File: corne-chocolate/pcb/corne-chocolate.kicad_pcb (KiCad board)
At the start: 2 copper layers, 133.8 x 91.4 mm, 98 parts, among them J3 LED, P1 i2c-pin, P2 i2c-pin, SW1 SW_PUSH, SW10 SW_PUSH, SW11 SW_PUSH, SW12 SW_PUSH, SW13 SW_PUSH, SW14 SW_PUSH, SW15 SW_PUSH, SW16 SW_PUSH, SW17 SW_PUSH, SW18 SW_PUSH, SW19 SW_PUSH, SW2 SW_PUSH, SW20 SW_PUSH, SW21 SW_PUSH, SW3 SW_PUSH, SW4 SW_PUSH, SW5 SW_PUSH, SW6 SW_PUSH, SW7 SW_PUSH, SW8 SW_PUSH, SW9 SW_PUSH, U1 ProMicro

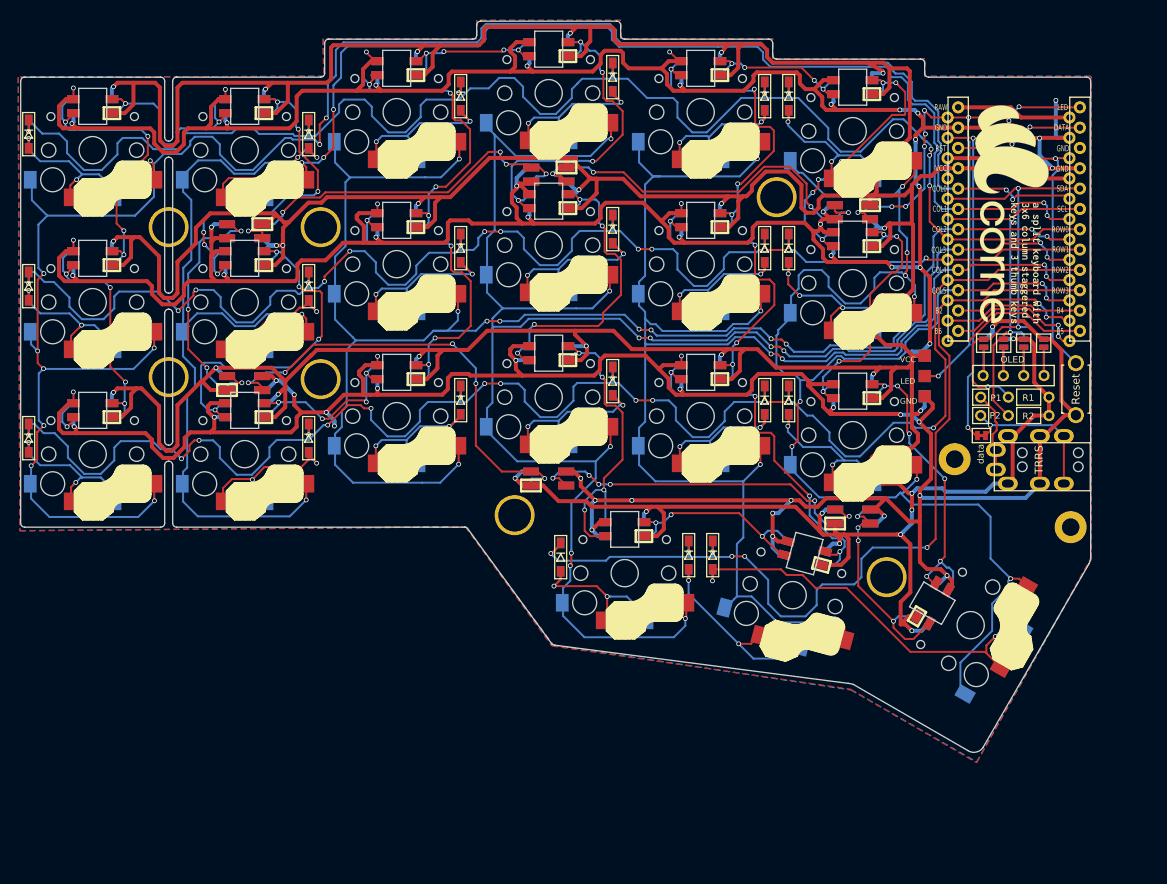
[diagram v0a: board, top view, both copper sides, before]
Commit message: rp2040 v0
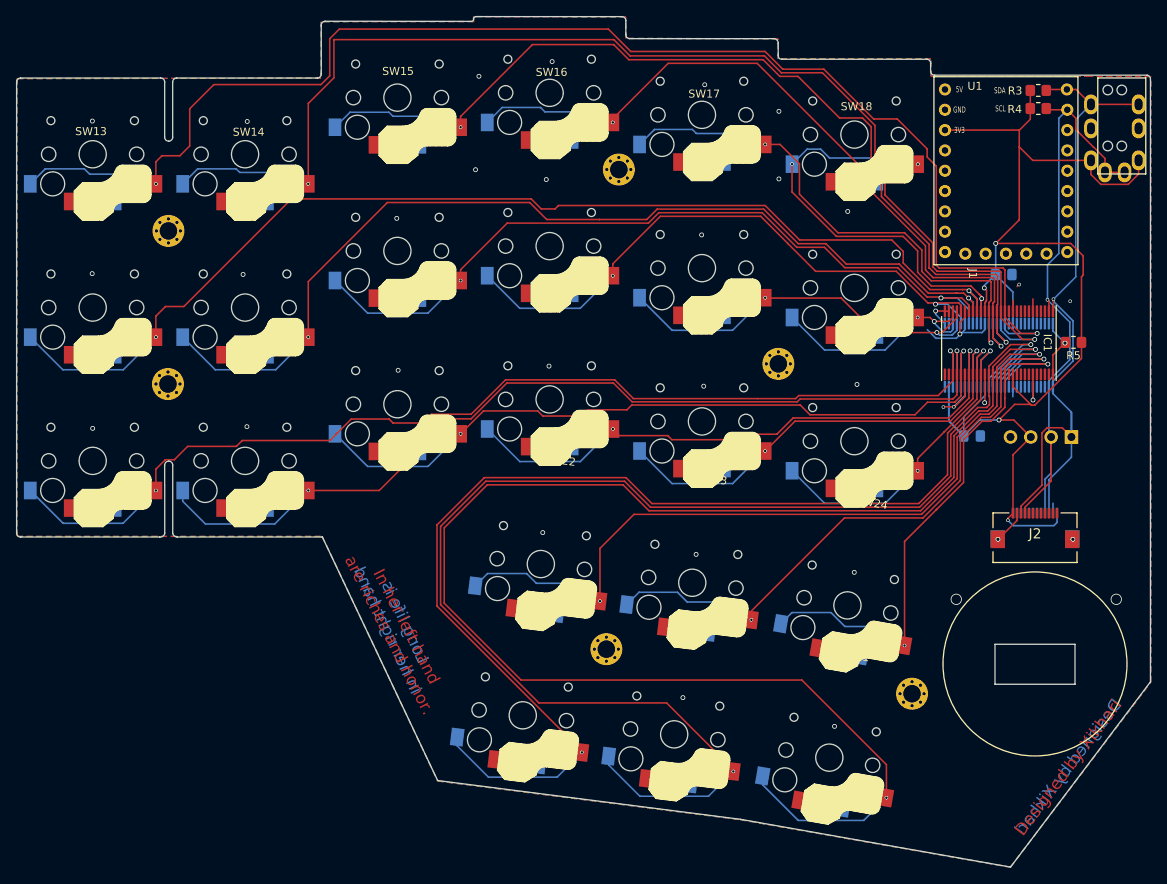
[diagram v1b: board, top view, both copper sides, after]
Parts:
- removed the ? at (79.5, 105.5)
- removed the ? at (177.8, 115.8)
- removed the ? at (192.2, 124.2)
- removed the ? at (79.5, 86.8)
- removed the ? at (98.5, 86.8)
- removed the ? at (98.5, 105.8)
- removed the ? at (155.5, 83.0)
- removed the ? at (122.8, 122.8)
- removed the ? at (169.2, 130.5)
- removed D1, D10, D11, D12, D13, D14, D15, D16, D17, D18, D19, D2, D20, D21, D3, D4, D5, D6, D7, D8, D9: D, kbd:D3_SMD
- removed G*** (x2): LOGO, kbd:corne
- removed JP2, JP3, JP4, JP5, JP6, JP7, JP8, JP9: , kbd:Jumper
- removed L1, L10, L11, L12, L13, L14, L15, L16, L17, L18, L19, L2, L20, L21, L3, L4, L5, L6, L7, L8, L9: SK6812MINI, kbd:SK6812MINI_rev
- removed L22, L23, L24, L25, L26, L27: SK6812MINI, kbd:SK6812MINI_underglow_rev
- removed OLED: OLED, kbd:OLED
- removed P1, P2: i2c-pin, kbd:1pin_conn
- removed R1, R2: R, kbd:R
- removed RSW1: Reset, kbd:ResetSW
- removed data: , kbd:JPC2
- added ?: , kbd:M2_HOLE_v3, F.Cu at (79.5, 87.2)
- added ?: , kbd:M2_HOLE_v3, F.Cu at (134.2, 139.5)
- added ?: , kbd:M2_HOLE_v3, F.Cu at (135.8, 79.5)
- added ?: , kbd:M2_HOLE_v3, F.Cu at (79.4, 106.4)
- added ?: , kbd:M2_HOLE_v3, F.Cu at (155.7, 103.8)
- added ?: , kbd:M2_HOLE_v3, F.Cu at (172.4, 145.1)
- added C1: 0.1uf, Capacitor_SMD:C_0805_2012Metric_Pad1.18x1.45mm_HandSolder, B.Cu at (183.9, 92.7)
- added C2: 0.1uf, Capacitor_SMD:C_0805_2012Metric_Pad1.18x1.45mm_HandSolder, B.Cu at (179.9, 112.9)
- added IC1: PCA9505, User-defined-footprints:TSSOP-56_7x14mm_P0.5mm_mr, F.Cu at (192.7, 102.0)
- added IC2: PCA9505, User-defined-footprints:TSSOP-56_7x14mm_P0.5mm_mr, B.Cu at (192.7, 102.0)
- added J2: FH12A-12S-0.5SH_55_, lib:FH12A12S05SH55, F.Cu at (187.8, 125.8)
- added J4: Conn_01x04_Male, Connector_PinHeader_2.54mm:PinHeader_1x04_P2.54mm_Vertical, B.Cu at (192.3, 113.0)
- added R3: 1k, Resistor_SMD:R_0805_2012Metric_Pad1.20x1.40mm_HandSolder, F.Cu at (188.2, 69.7)
- added R4: 1k, Resistor_SMD:R_0805_2012Metric_Pad1.20x1.40mm_HandSolder, F.Cu at (188.2, 71.9)
- added R5: 1k, Resistor_SMD:R_0805_2012Metric_Pad1.20x1.40mm_HandSolder, F.Cu at (192.6, 101.2)
- added SW22: SW_PUSH, User-defined-footprints:kbd-switches, F.Cu at (127.1, 119.3)
- added SW23: SW_PUSH, User-defined-footprints:kbd-switches, F.Cu at (146.0, 121.7)
- added SW24: SW_PUSH, User-defined-footprints:kbd-switches, F.Cu at (165.9, 124.6)
- J1: renamed from TRRS; footprint kbd:MJ-4PP-9 -> User-defined-footprints:4-ring-jack-mr
- J3: value LED -> FH12A-12S-0.5SH_55_; footprint kbd:StripLED_rev -> lib:FH12A12S05SH55; moved to B.Cu
- SW1, SW10, SW11, SW12, SW13, SW14, SW15, SW16, SW17, SW18, SW19, SW2, SW20, SW3, SW4, SW5, SW6, SW7, SW8, SW9: footprint kbd:Choc_Hotswap -> User-defined-footprints:kbd-switches
- SW21: footprint kbd:Choc_Hotswap_1.5u -> User-defined-footprints:kbd-switches
- U1: value ProMicro -> waveshare-rp2040-zero; footprint kbd:ProMicro_v2 -> User-defined-footprints:rp2040-zero-mr
- moved SW15 49.4 mm to (108.0, 61.0), turned to 0 degrees
- moved SW16 47.6 mm to (127.0, 60.4), turned to 0 degrees
- moved SW17 47.2 mm to (146.1, 63.1), turned to 0 degrees
- moved SW18 47.1 mm to (165.1, 65.6), turned to 0 degrees
- moved SW13 47.1 mm to (69.9, 68.1), turned to 0 degrees
- moved SW14 47.1 mm to (89.0, 68.1), turned to 0 degrees
- moved J1 42.4 mm to (191.1, 74.5), turned to 90 degrees
- moved SW1 29.3 mm to (69.9, 106.4), turned to 0 degrees
- moved SW2 29.3 mm to (89.0, 106.4), turned to 0 degrees
- moved SW6 29.2 mm to (165.1, 103.9), turned to 0 degrees
- moved SW5 29.1 mm to (146.1, 101.5), turned to 0 degrees
- moved SW4 28.7 mm to (127.0, 98.7), turned to 0 degrees
- moved SW3 26.9 mm to (108.0, 99.3), turned to 0 degrees
- moved J3 22.5 mm to (187.8, 125.7)
- moved U1 21.1 mm to (175.2, 67.9)
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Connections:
- J1 pad A: Net-(J1-PadA) -> SCL0
- J1 pad B: Net-(J1-PadB) -> SDA0
- J3 pad 1: GND -> VCC
- J3 pad 2: LED -> GND
- J3 pad 3: VCC -> SDA0
- SW1 pad 1: col0 -> 1r5
- SW1 pad 2: Net-(D1-Pad2) -> GND
- SW10 pad 1: col3 -> 2r2
- SW10 pad 2: Net-(D10-Pad2) -> GND
- SW11 pad 1: col4 -> 2r1
- SW11 pad 2: Net-(D11-Pad2) -> GND
- SW12 pad 1: col5 -> 2r0
- SW12 pad 2: Net-(D12-Pad2) -> GND
- SW13 pad 1: col0 -> 0r5
- SW13 pad 2: Net-(D13-Pad2) -> GND
- SW14 pad 1: col1 -> 0r4
- SW14 pad 2: Net-(D14-Pad2) -> GND
- SW15 pad 1: col2 -> 0r3
- SW15 pad 2: Net-(D15-Pad2) -> GND
- SW16 pad 1: col3 -> 0r2
- SW16 pad 2: Net-(D16-Pad2) -> GND
- SW17 pad 1: col4 -> 0r1
- SW17 pad 2: Net-(D17-Pad2) -> GND
- SW18 pad 1: col5 -> 0r0
- SW18 pad 2: Net-(D18-Pad2) -> GND
- SW19 pad 1: col3 -> 3r5
- SW19 pad 2: Net-(D19-Pad2) -> GND
- SW2 pad 1: col1 -> 1r4
- SW2 pad 2: Net-(D2-Pad2) -> GND
- SW20 pad 1: col4 -> 3r4
- SW20 pad 2: Net-(D20-Pad2) -> GND
- SW21 pad 1: col5 -> 3r3
- SW21 pad 2: Net-(D21-Pad2) -> GND
- SW3 pad 1: col2 -> 1r3
- SW3 pad 2: Net-(D3-Pad2) -> GND
- SW4 pad 1: col3 -> 1r2
- SW4 pad 2: Net-(D4-Pad2) -> GND
- SW5 pad 1: col4 -> 1r1
- SW5 pad 2: Net-(D5-Pad2) -> GND
- SW6 pad 1: col5 -> 1r0
- SW6 pad 2: Net-(D6-Pad2) -> GND
- SW7 pad 1: col0 -> 2r5
- SW7 pad 2: Net-(D7-Pad2) -> GND
- SW8 pad 1: col1 -> 2r4
- SW8 pad 2: Net-(D8-Pad2) -> GND
- SW9 pad 1: col2 -> 2r3
- SW9 pad 2: Net-(D9-Pad2) -> GND
- U1 pad 1: LED -> SCL0
- U1 pad 10: row3 -> unconnected-(U1-Pad10)
- U1 pad 11: Net-(U1-Pad11) -> unconnected-(U1-Pad11)
- U1 pad 12: Net-(U1-Pad12) -> unconnected-(U1-Pad12)
- U1 pad 13: Net-(U1-Pad13) -> unconnected-(U1-Pad13)
- U1 pad 14: Net-(U1-Pad14) -> unconnected-(U1-Pad14)
- U1 pad 15: col5 -> unconnected-(U1-Pad15)
- U1 pad 16: col4 -> unconnected-(U1-Pad16)
- U1 pad 17: col3 -> unconnected-(U1-Pad17)
- U1 pad 18: col2 -> unconnected-(U1-Pad18)
- U1 pad 19: col1 -> unconnected-(U1-Pad19)
- U1 pad 2: data -> unconnected-(U1-Pad2)
- U1 pad 20: col0 -> VCC
- U1 pad 21: VCC -> GND
- U1 pad 22: reset -> unconnected-(U1-Pad22)
- U1 pad 3: GND -> unconnected-(U1-Pad3)
- U1 pad 4: GND -> unconnected-(U1-Pad4)
- U1 pad 5: SDA -> unconnected-(U1-Pad5)
- U1 pad 6: SCL -> unconnected-(U1-Pad6)
- U1 pad 7: row0 -> unconnected-(U1-Pad7)
- U1 pad 8: row1 -> unconnected-(U1-Pad8)
- U1 pad 9: row2 -> unconnected-(U1-Pad9)
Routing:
- net GND: track 816.7 -> 46.2 mm, vias 59 -> 35
- net VCC: track 786.4 -> 153.5 mm, vias 30 -> 4
- net col0: track 255.1 -> 0.00 mm, vias 12 -> 0
- net col1: track 232.6 -> 0.00 mm, vias 7 -> 0
- net col3: track 224.8 -> 0.00 mm, vias 12 -> 0
- net row2: track 209.9 -> 0.00 mm, vias 15 -> 0
- net row0: track 197.4 -> 0.00 mm, vias 9 -> 0
- net 3r3: track 0.00 -> 196.4 mm, vias 0 -> 2
- net col4: track 196.2 -> 0.00 mm, vias 8 -> 0
- net col2: track 193.4 -> 0.00 mm, vias 11 -> 0
- net col5: track 188.2 -> 0.00 mm, vias 10 -> 0
- net row1: track 187.4 -> 0.00 mm, vias 15 -> 0
- net 0r5: track 0.00 -> 175.1 mm, vias 0 -> 2
- net 3r4: track 0.00 -> 174.6 mm, vias 0 -> 2
- net 0r4: track 0.00 -> 155.1 mm, vias 0 -> 2
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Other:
- board size 133.8 x 91.4 mm -> 141.7 x 106.3 mm
- net class Default removed
- board text added: "Designed by Xikhari"
- board text added: "In her left hand are riches and honor."
- board text added: "JLCJLCJLCJLC"
- board text added: "Long life is in her right hand"
- board text removed: "Corne Chocolate v2.1 PCB designed by foostan"
- board text removed: "GND"
- board text removed: "LED"
- board text removed: "OLED"
- board text removed: "VCC"
